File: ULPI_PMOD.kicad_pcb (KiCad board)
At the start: 2 copper layers, 16 parts, among them P1 CONN_01X02, P2 USB_OTG, P3 JB, P4 JC, U1 STMPS2141, U2 USB3300, Y1 Crystal

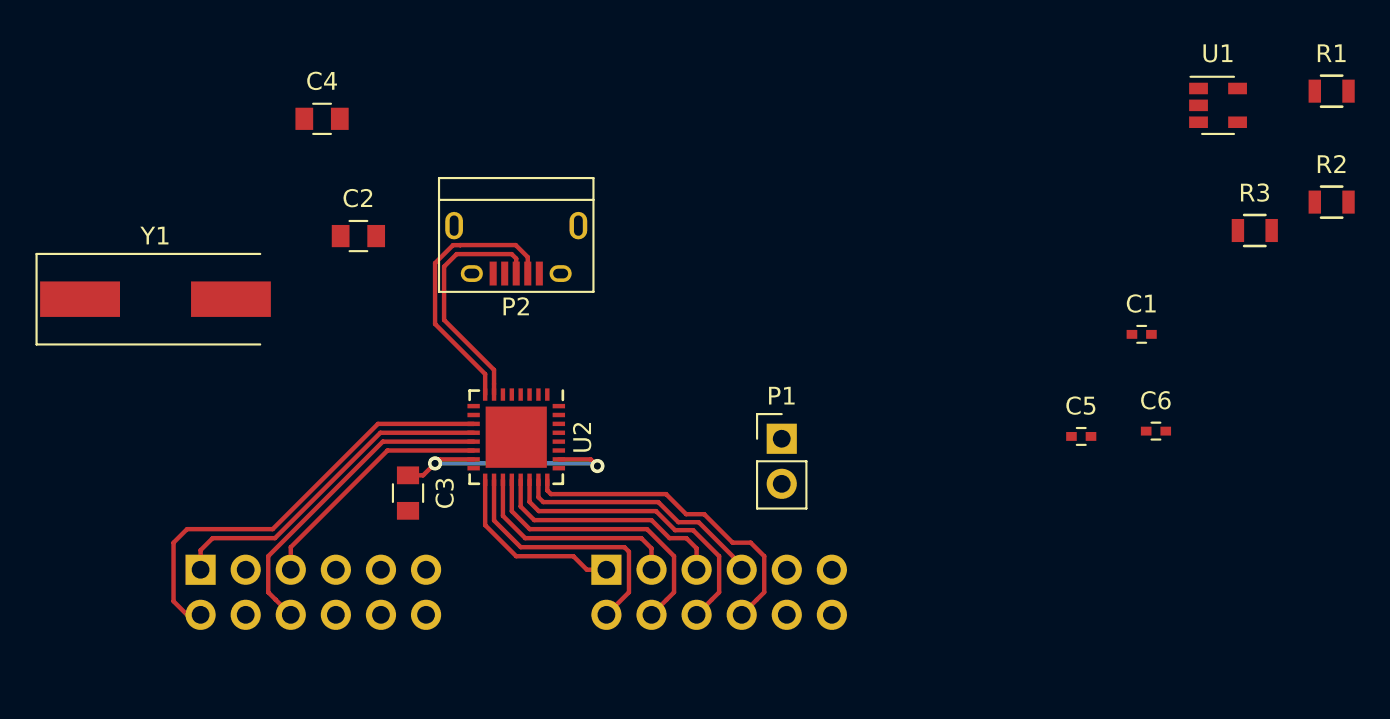
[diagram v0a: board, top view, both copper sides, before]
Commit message: PCB done.
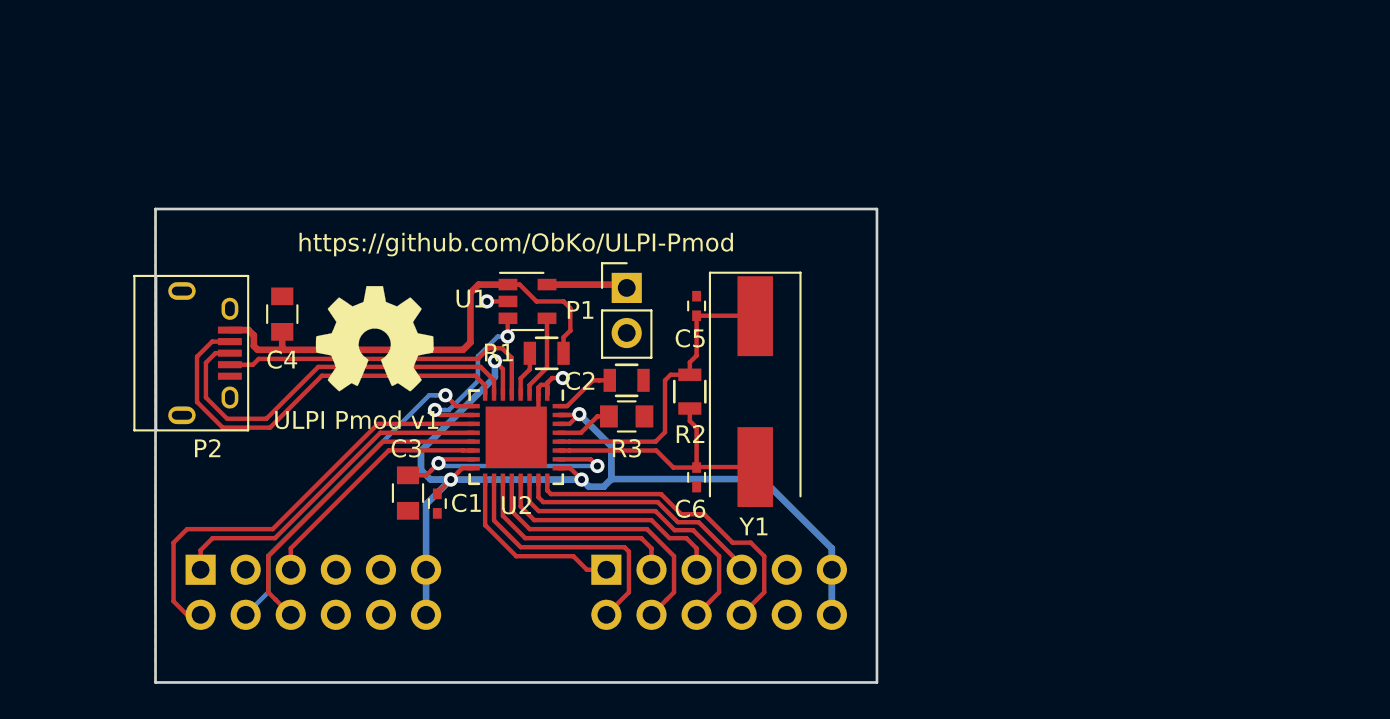
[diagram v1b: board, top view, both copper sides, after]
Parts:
- added REF***: OSHW-Symbol_6.7x6mm_SilkScreen, Symbols:OSHW-Symbol_6.7x6mm_SilkScreen, F.Cu at (86.0, 63.2)
- moved R1 46.6 mm to (95.7, 64.0)
- moved C1 40.8 mm to (89.5, 72.5), turned to 270 degrees
- moved U1 40.4 mm to (94.6, 61.1)
- moved R2 37.7 mm to (103.8, 66.2), turned to 90 degrees
- moved R3 36.4 mm to (100.2, 65.5)
- moved Y1 34.2 mm to (107.4, 66.2), turned to 270 degrees
- moved C6 26.0 mm to (104.1, 71.0), turned to 270 degrees
- moved C5 22.9 mm to (104.1, 61.3), turned to 90 degrees
- moved P2 18.4 mm to (76.5, 64.0), turned to 270 degrees
- moved C2 18.2 mm to (100.2, 67.6)
- moved P1 12.2 mm to (100.2, 60.3)
- moved C4 11.2 mm to (80.8, 61.8), turned to 90 degrees
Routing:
- net +3V3: track 0.00 -> 59.0 mm, vias 0 -> 4
- net Net-(C4-Pad1): track 0.00 -> 27.4 mm
- net /ULPI_RESET: track 0.00 -> 19.4 mm, vias 0 -> 1
- net Net-(P2-Pad4): track 0.00 -> 18.6 mm
- net Net-(C5-Pad1): track 0.00 -> 17.5 mm
- net Net-(C6-Pad1): track 0.00 -> 15.0 mm
- net /EXTVBUS: track 0.00 -> 9.96 mm, vias 0 -> 2
- net /D+: track 13.7 -> 22.6 mm
- net /D-: track 15.4 -> 23.5 mm
- net GND: track 0.00 -> 5.98 mm, vias 0 -> 2
- net /CPEN: track 0.00 -> 4.70 mm
- net +5V: track 0.00 -> 4.57 mm
- net Net-(R3-Pad1): track 0.00 -> 3.47 mm
- net Net-(C2-Pad1): track 0.00 -> 3.20 mm
- net Net-(R1-Pad1): track 0.00 -> 2.54 mm
- added copper zone on B.Cu, net GND
- added copper zone on F.Cu, net GND
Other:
- board outline added: 40.6 x 26.7 mm
- board text added: "ULPI Pmod v1"
- board text added: "https://github.com/ObKo/ULPI-Pmod"
